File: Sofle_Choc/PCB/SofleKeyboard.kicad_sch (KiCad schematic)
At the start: 110 parts, among them J2 4PIN, J3 OLED, P1 i2c_pin, P2 i2c_pin, SW1 SW_PUSH_LED, SW10 SW_PUSH_LED, SW11 SW_PUSH_LED, SW12 SW_PUSH_LED, SW13 SW_PUSH_LED, SW14 SW_PUSH_LED, SW15 SW_PUSH_LED, SW16 SW_PUSH_LED, SW17 SW_PUSH_LED, SW18 SW_PUSH_LED, SW19 SW_PUSH_LED, SW2 SW_PUSH_LED, SW20 SW_PUSH_LED, SW21 SW_PUSH_LED, SW22 SW_PUSH_LED, SW23 SW_PUSH_LED, SW24 SW_PUSH_LED, SW25 Rotary_Encoder_Switch, SW26 SW_PUSH_LED, SW27 SW_PUSH_LED, SW28 SW_PUSH_LED, SW29 SW_PUSH_LED, SW3 SW_PUSH_LED, SW30 SW_PUSH_LED, SW31 SW_PUSH_LED, SW32 SW_PUSH_LED, SW33 SW_PUSH_LED, SW4 SW_PUSH_LED, SW5 SW_PUSH_LED, SW6 SW_PUSH_LED, SW7 SW_PUSH_LED, SW8 SW_PUSH_LED, SW9 SW_PUSH_LED, U1 ProMicro

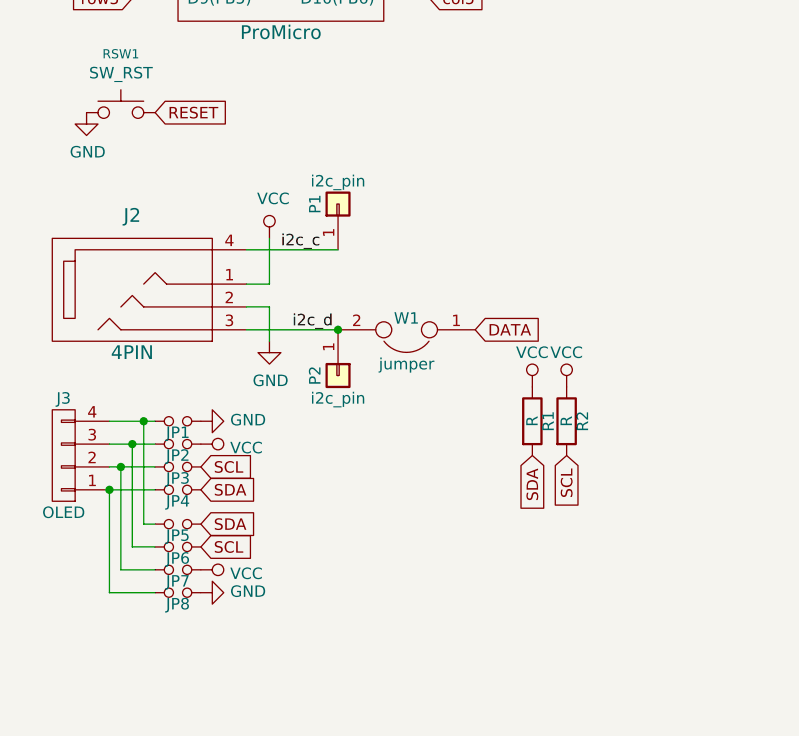
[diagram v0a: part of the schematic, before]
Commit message: Cleanup
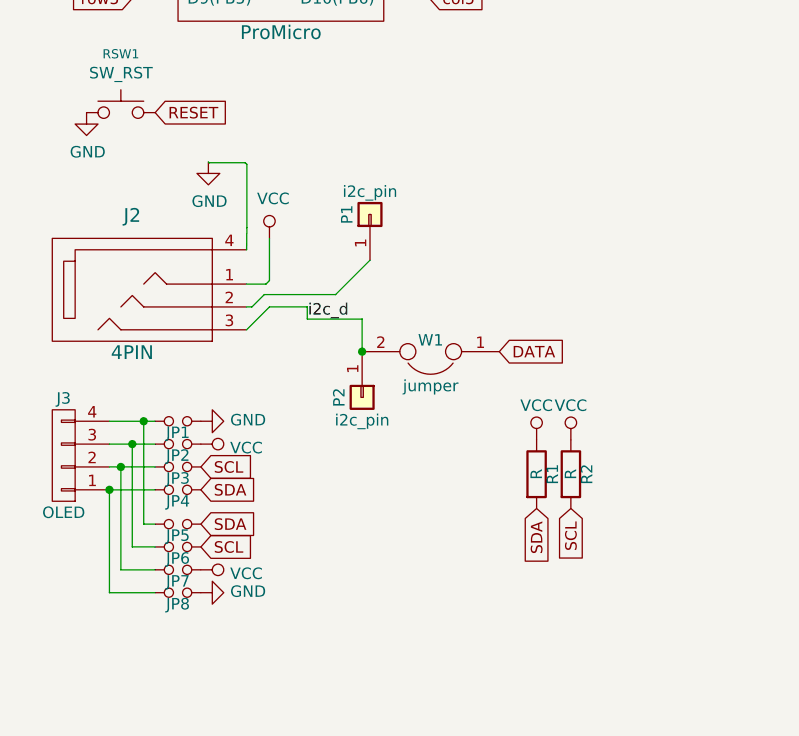
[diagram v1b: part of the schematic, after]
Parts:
- J2: footprint SofleKeyboard-footprint:MJ-4PP-9 -> SofleChoc:3.5mm_6_contacts_4_conductors_audio_plug
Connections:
- net GND: now also J2.4; no longer J2.2
- net i2c_c: no longer names the net of P1.1 (Pin_1)
- net i2c_c: now also J2.2; no longer J2.4
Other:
- moved on the sheet: P1, P2, R1, R2, W1
